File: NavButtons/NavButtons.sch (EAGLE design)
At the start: 11 parts

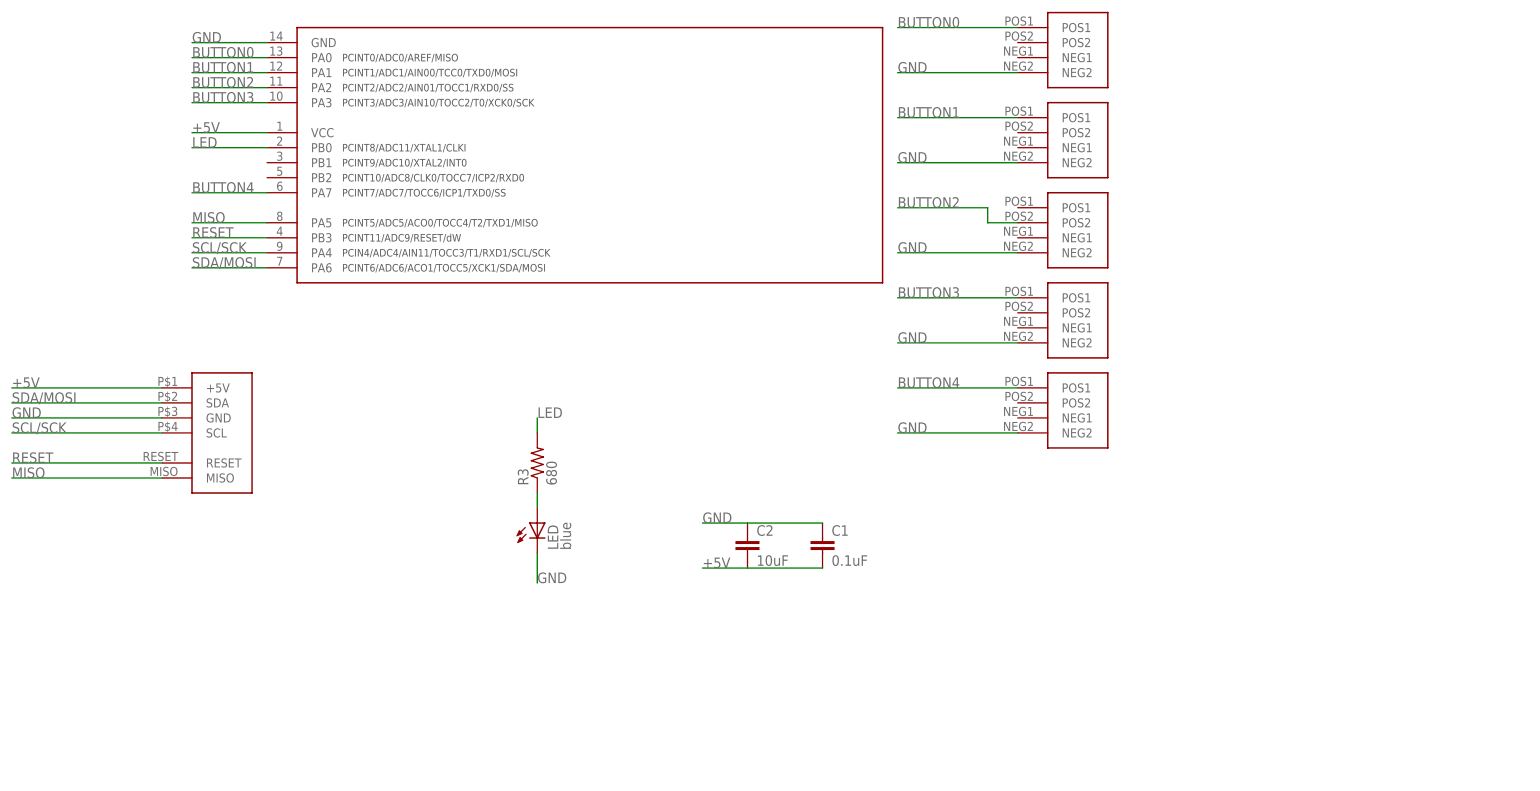
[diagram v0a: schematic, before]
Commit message: Latest version of schematics and boards
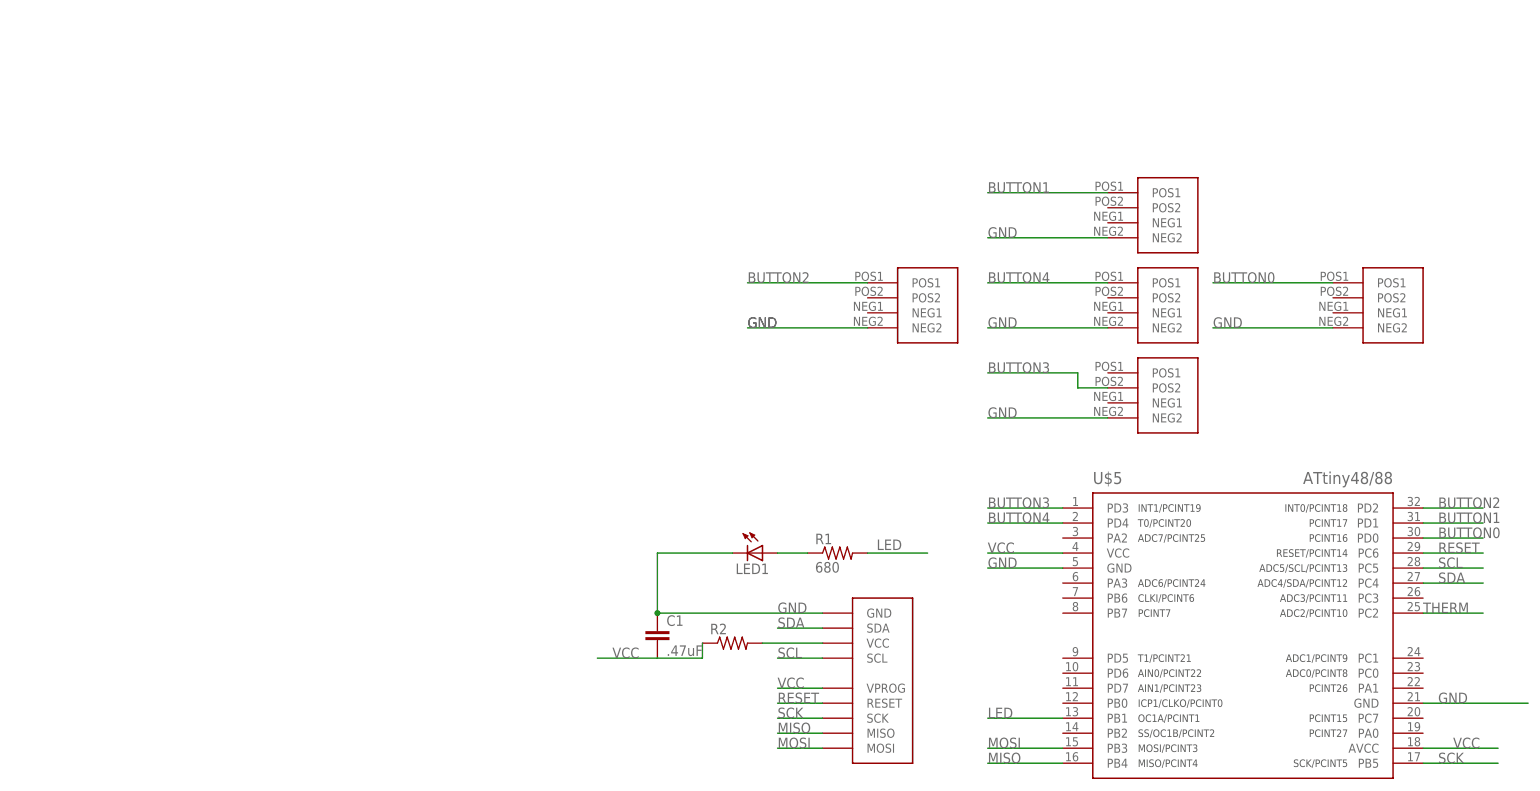
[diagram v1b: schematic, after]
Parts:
- removed C2: 10uF, SparkFun-Capacitors:CAP0805
- removed LED: blue, led:LEDCHIPLED_1206
- removed R3: 680, SparkFun-Passives:RESISTOR0805-RES
- removed U$1, U$6, U$7, U$8: TACT-SWITCH, IntegerLabs:TACT-SWITCH
- removed U$3: TINY841, IntegerLabs:TINY841
- removed U$4: FOOTPRINT, IntegerLabs:FOOTPRINT
- added B1, B3, B4, B5, B7: TACT-SWITCH, IntegerLabs:TACT-SWITCH
- added LED1: (no value), adafruit:LEDCHIP-LED0805
- added R1: 680, SparkFun-Passives:RESISTOR0805-RES
- added R2: (no value), SparkFun-Resistors:RESISTOR0805-RES
- added U$5: ATTINY48/88-TQFP, IntegerLabs:ATTINY48/88-TQFP
- C1: value 0.1uF -> .47uF
- U$2: value TACT-SWITCH -> FOOTPRINTFOOTPRINT-2; device IntegerLabs:TACT-SWITCH -> IntegerLabs:FOOTPRINTFOOTPRINT-2
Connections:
- removed net +5V: C1.2, C2.2, U$3.VCC, U$4.+5V
- removed net N$5: LED.A, R3.1
- removed net SCL/SCK: U$3.PA4, U$4.SCL
- removed net SDA/MOSI: U$3.PA6, U$4.SDA
- new net MOSI: U$2.MOSI, U$5.PB3
- new net N$2: R2.2, U$2.VCC
- new net N$8: LED1.A, R1.1
- new net SCK: U$2.SCK, U$5.PB5
- new net SCL: U$2.SCL, U$5.PC5
- new net SDA: U$2.SDA, U$5.PC4
- new net THERM: U$5.PC2
- new net VCC: C1.2, R2.1, U$2.VPROG, U$5.VCC
- net BUTTON0: now also B5.POS1, U$5.PD0; no longer U$1.POS1, U$3.PA0
- net BUTTON1: now also B1.POS1, U$5.PD1; no longer U$2.POS1, U$3.PA1
- net BUTTON2: now also B3.POS1, U$5.PD2; no longer U$3.PA2, U$6.POS2
- net BUTTON3: now also B7.POS2, U$5.PD3; no longer U$3.PA3, U$7.POS1
- net BUTTON4: now also B4.POS1, U$5.PD4; no longer U$3.PA7, U$8.POS1
- net GND: now also B1.NEG2, B3.NEG2, B4.NEG2, B5.NEG2, B7.NEG2, LED1.C, U$2.GND, U$5.GND, U$5.GND@1; no longer C2.1, LED.C, U$1.NEG2, U$2.NEG2, U$3.GND, U$4.GND, U$6.NEG2, U$7.NEG2, U$8.NEG2
- net LED: now also R1.2, U$5.PB1; no longer R3.2, U$3.PB0
- net MISO: now also U$2.MISO, U$5.PB4; no longer U$3.PA5, U$4.MISO
- net RESET: now also U$2.RESET, U$5.PC6; no longer U$3.PB3, U$4.RESET
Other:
- moved on the sheet: C1
